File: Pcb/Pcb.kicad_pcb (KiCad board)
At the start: 2 copper layers, 152.3 x 104.7 mm, 130 parts, among them J1 TRRS, Q1 2N7002, SW1 SW_Push, SW10 SW_Push, SW11 SW_Push, SW12 SW_Push, SW13 SW_Push, SW14 SW_Push, SW15 SW_Push, SW16 SW_Push, SW17 SW_Push, SW18 SW_Push, SW19 SW_Push, SW2 SW2, SW20 SW_Push, SW21 SW_Push, SW22 SW_Push, SW23 SW_Push, SW24 SW_Push, SW25 SW_Push, SW26 SW_Push, SW27 SW_Push, SW28 SW_Push, SW29 SW_Push, SW3 SW_Push, SW4 SW_Push, SW5 SW_Push, SW6 SW_Push, SW7 SW_Push, SW8 SW_Push, SW9 SW_Push, U1 ProMicro

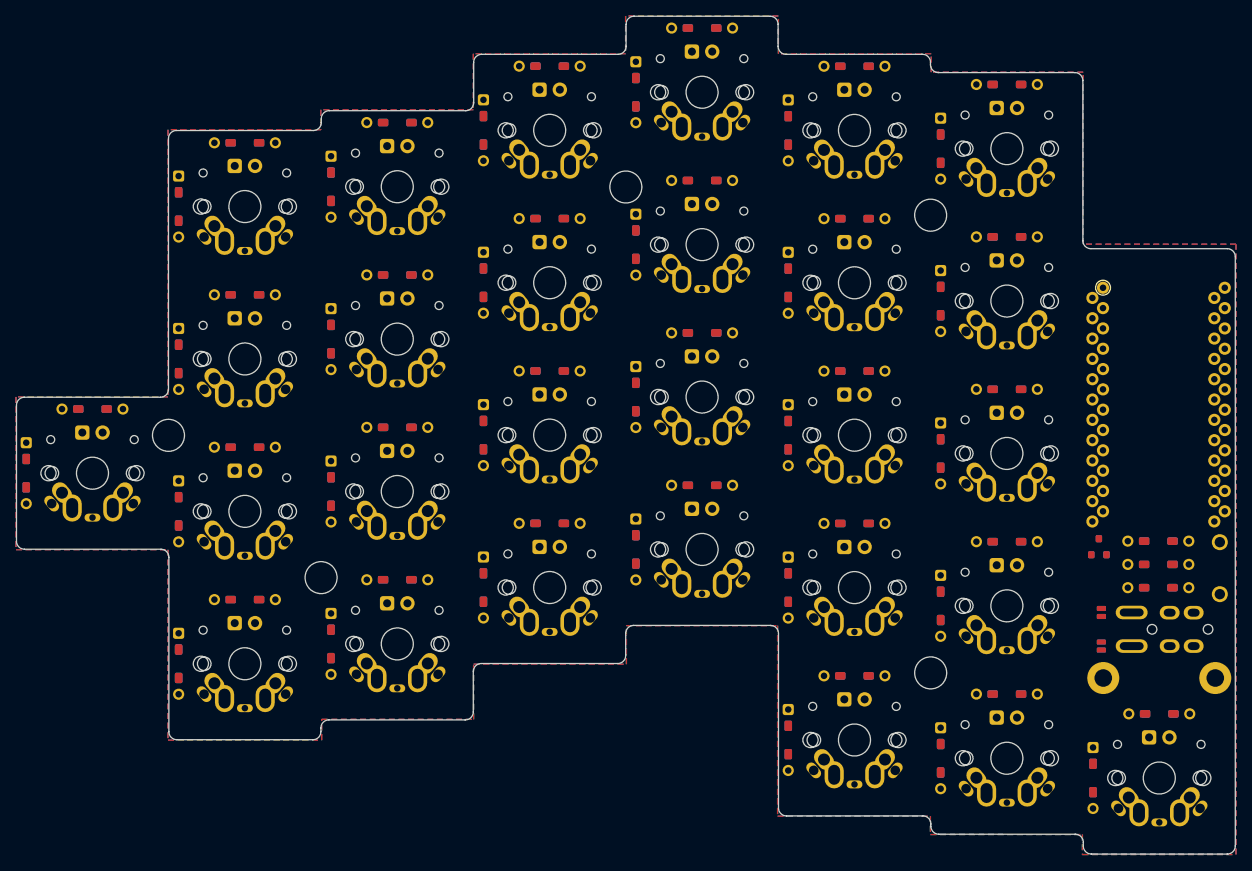
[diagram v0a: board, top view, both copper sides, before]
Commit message: Route tracks
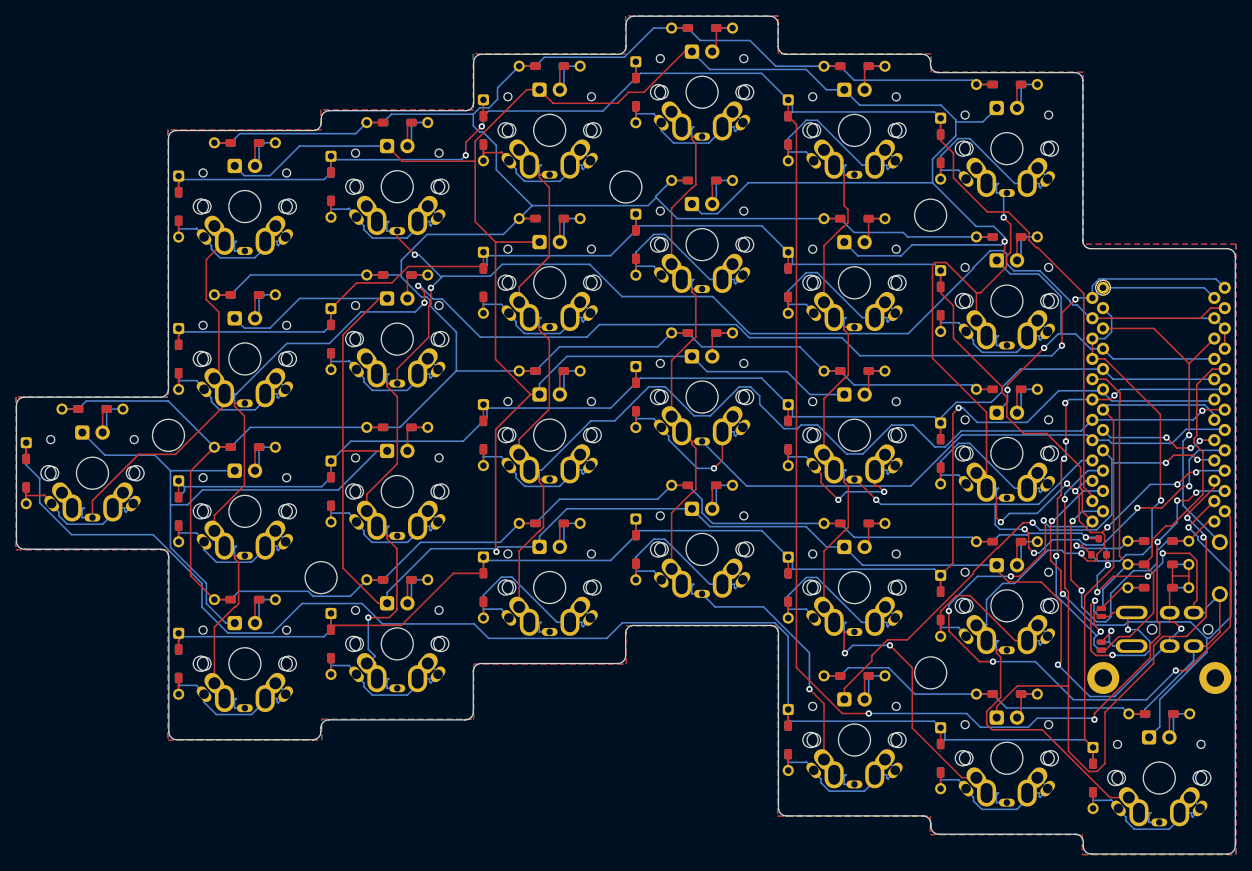
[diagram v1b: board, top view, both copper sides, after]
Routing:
- net VCC: track 0.00 -> 628.5 mm, vias 0 -> 6
- net /LEDOut: track 0.00 -> 573.1 mm, vias 0 -> 1
- net /rowA: track 0.00 -> 331.1 mm, vias 0 -> 7
- net /col0: track 0.00 -> 259.0 mm, vias 0 -> 4
- net /rowB: track 0.00 -> 249.8 mm, vias 0 -> 5
- net /rowE: track 0.00 -> 237.2 mm
- net /col1: track 0.00 -> 202.2 mm, vias 0 -> 3
- net /col4: track 0.00 -> 195.9 mm, vias 0 -> 7
- net /col5: track 0.00 -> 191.7 mm, vias 0 -> 8
- net /col3: track 0.00 -> 188.4 mm, vias 0 -> 1
- net /col2: track 0.00 -> 185.0 mm, vias 0 -> 1
- net /rowD: track 0.00 -> 182.8 mm, vias 0 -> 1
- net GND: track 0.00 -> 164.3 mm, vias 0 -> 5
- net /rowC: track 0.00 -> 163.4 mm
- net /SCROLL: track 0.00 -> 100.5 mm, vias 0 -> 3
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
